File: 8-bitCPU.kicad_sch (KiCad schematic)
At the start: 0 parts

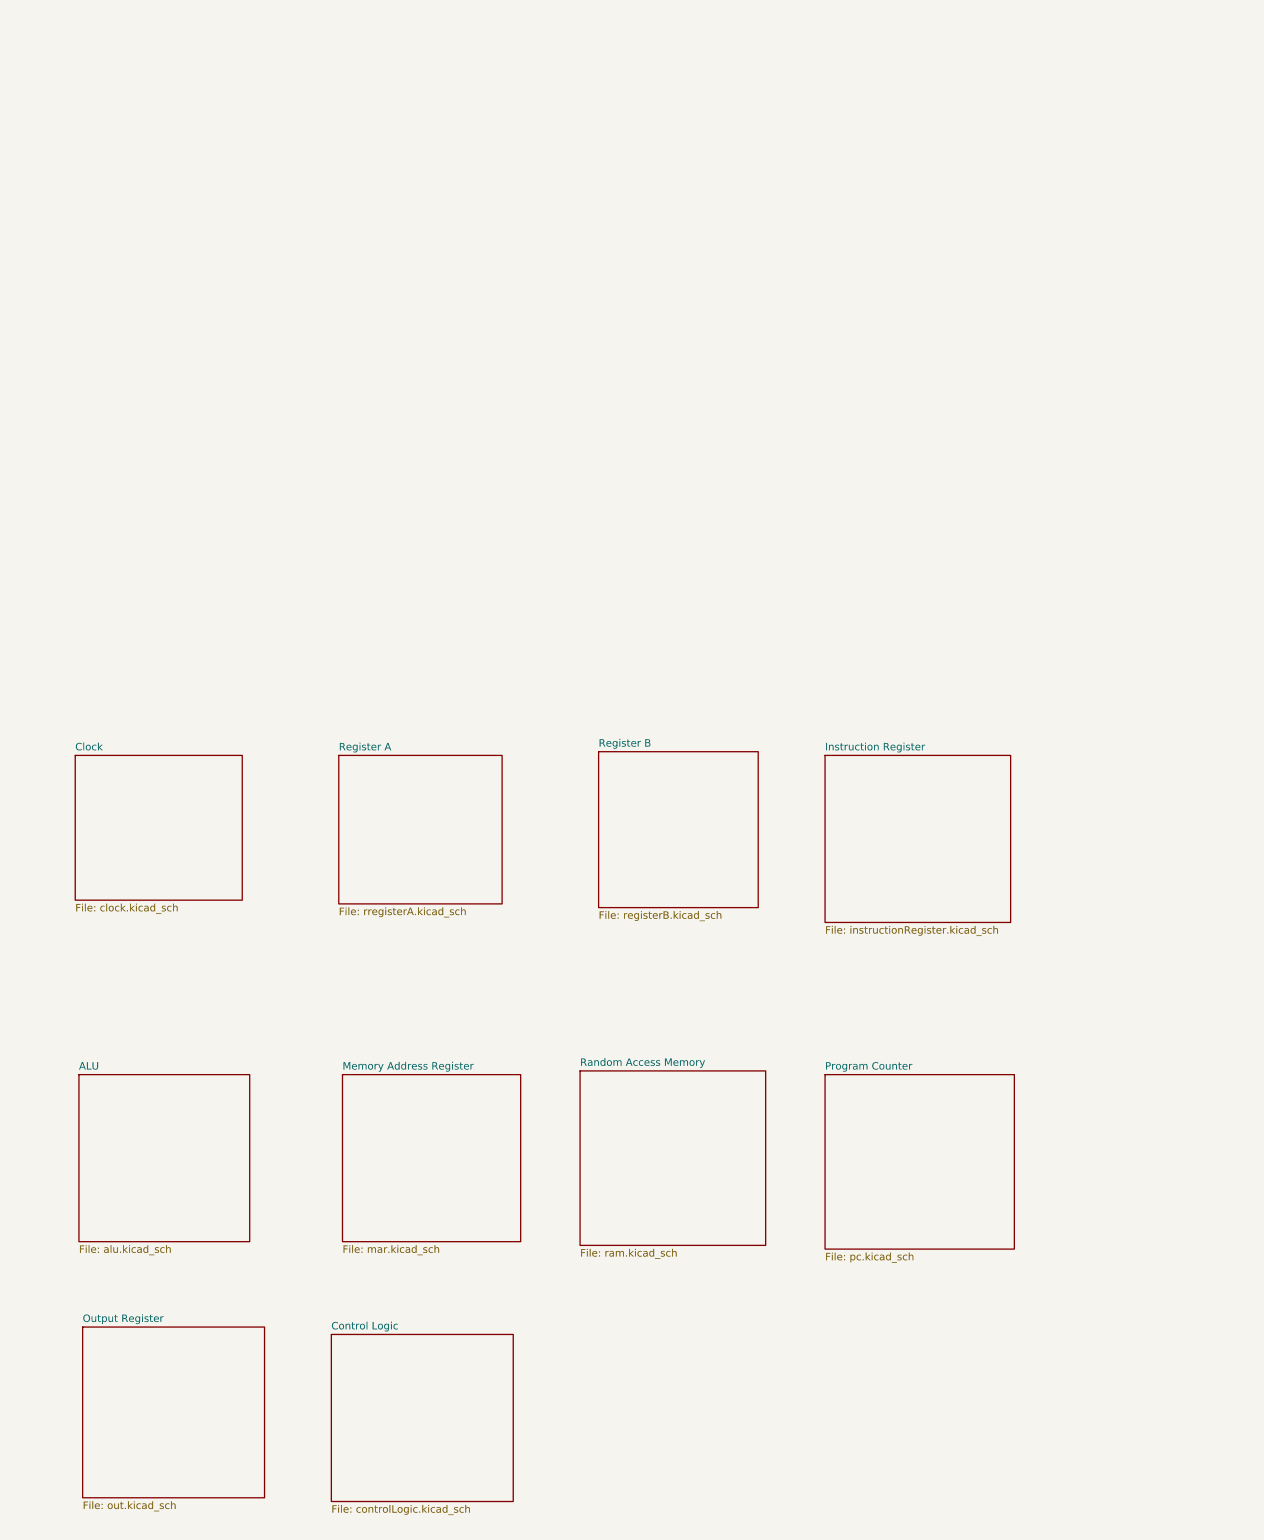
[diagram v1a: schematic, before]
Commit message: Alu & Mar
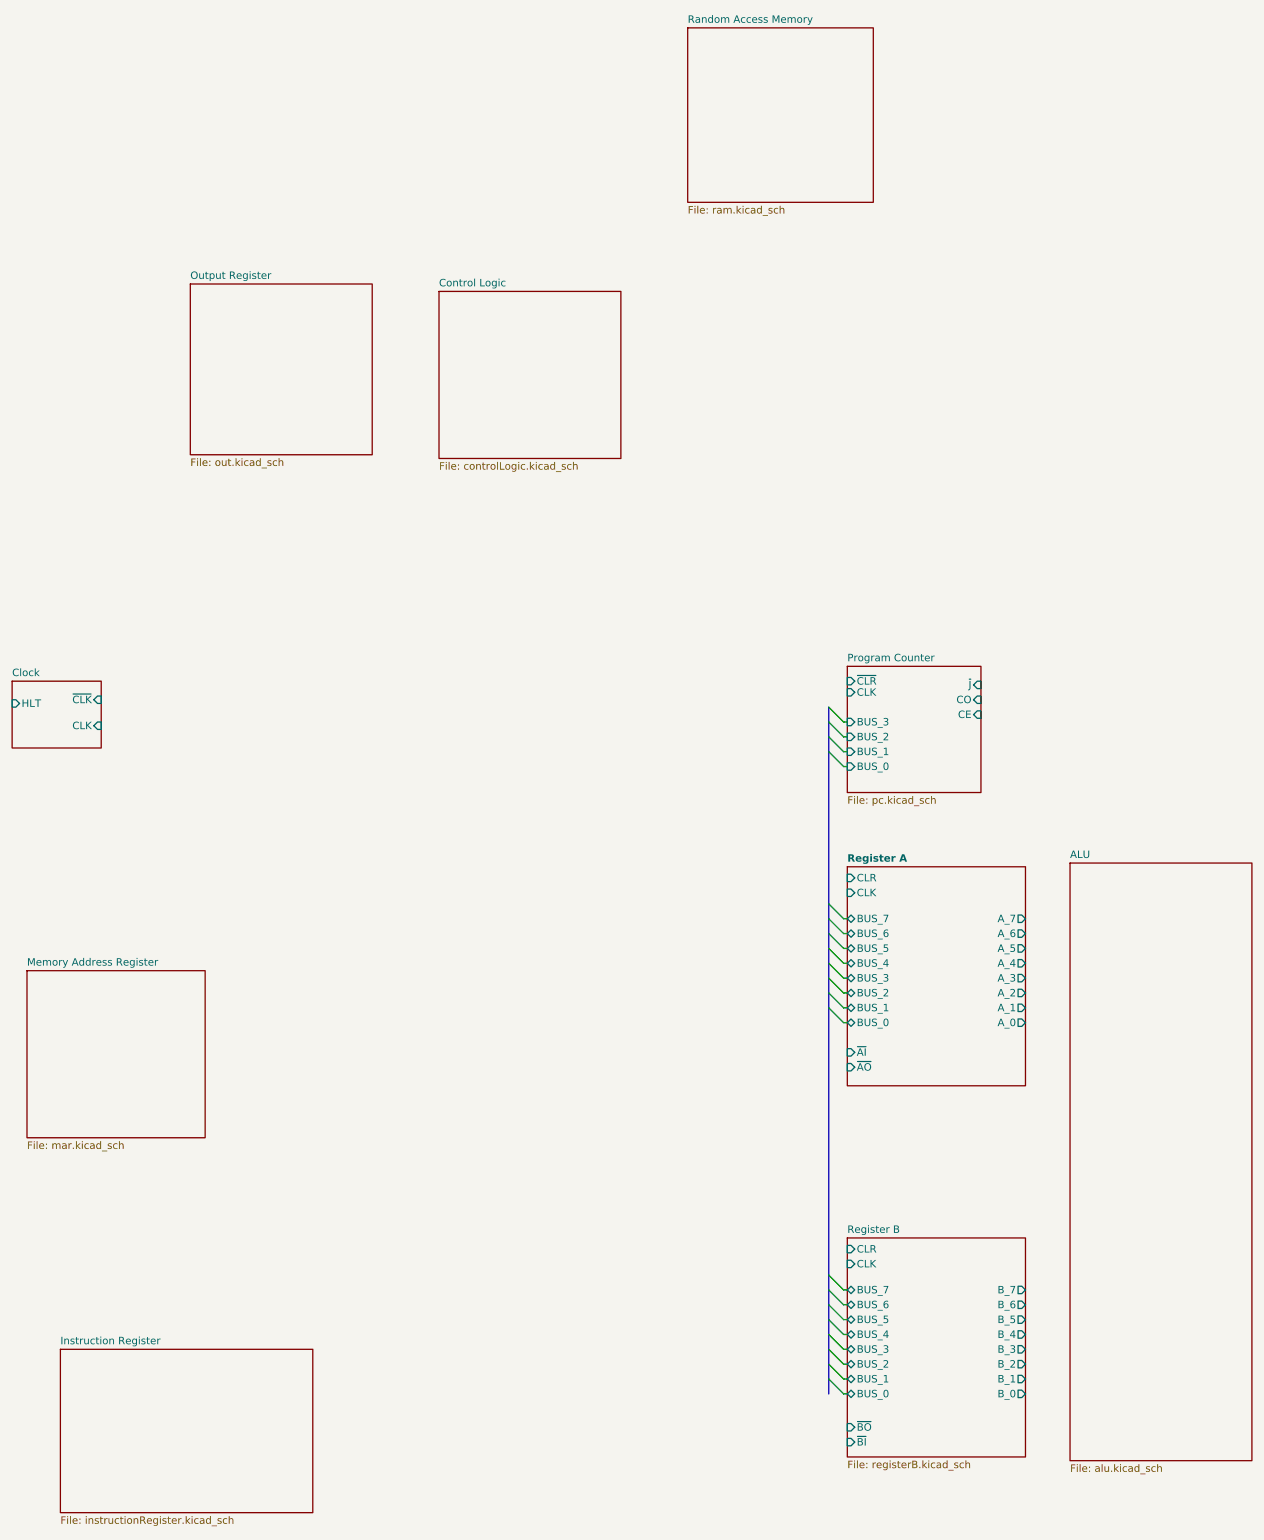
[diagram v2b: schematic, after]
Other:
- sheet Clock ports: added CLK, HLT, ~{CLK}; removed none
- sheet Program Counter ports: added BUS_0, BUS_1, BUS_2, BUS_3, CE, CLK, CO, ~{CLR}, ~{J}; removed none
- sheet Register A: file rregisterA.kicad_sch -> registerA.kicad_sch
- sheet Register A ports: added A_0, A_1, A_2, A_3, A_4, A_5, A_6, A_7, BUS_0, BUS_1, BUS_2, BUS_3, BUS_4, BUS_5, BUS_6, BUS_7, CLK, CLR, ~{AI}, ~{AO}; removed none
- sheet Register B ports: added BUS_0, BUS_1, BUS_2, BUS_3, BUS_4, BUS_5, BUS_6, BUS_7, B_0, B_1, B_2, B_3, B_4, B_5, B_6, B_7, CLK, CLR, ~{BI}, ~{BO}; removed none
